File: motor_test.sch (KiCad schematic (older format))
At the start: 41 parts, among them J1 Conn_01x02_Male, J2 Conn_01x01_Male, J3 Conn_01x01_Male, J4 Conn_01x02_Male, Q1 BC817, Q10 FR024N, Q11 BC807, Q12 BC817, Q13 BC817, Q14 BC817, Q15 BC807, Q16 BC817, Q2 BC817, Q3 BC807, Q4 BC817, Q5 BC807, Q6 BC817, Q7 FR9024N, Q8 FR024N, Q9 FR9024N

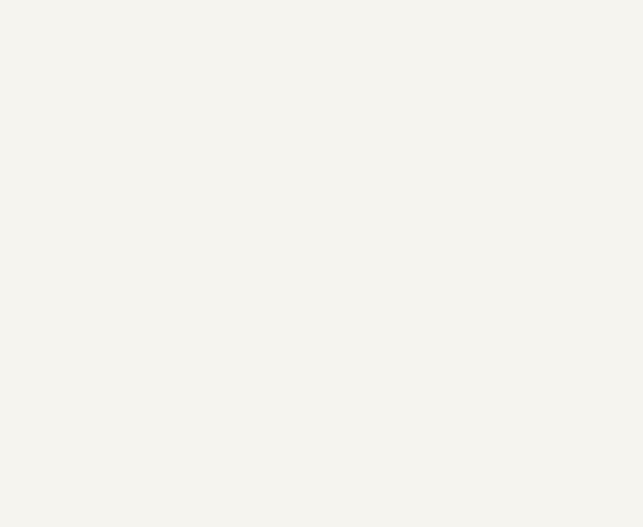
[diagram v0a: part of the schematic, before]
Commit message: bistable
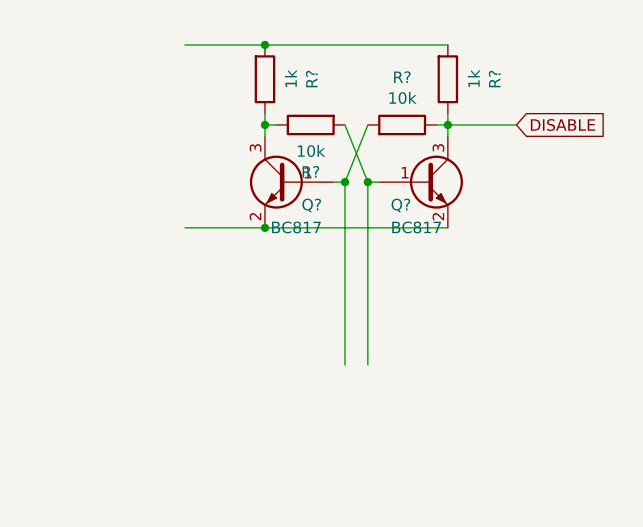
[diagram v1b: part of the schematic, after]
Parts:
- added Q? (x2): BC817, Package_TO_SOT_SMD:SOT-23, symbol Transistor_BJT:BC817
- added R? (x2): 1k, Resistor_SMD:R_1206_3216Metric, symbol Device:R
- added R? (x2): 10k, Resistor_SMD:R_1206_3216Metric, symbol Device:R
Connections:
- wire segments 119 -> 136
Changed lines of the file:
@@
 Wire Wire Line
 	1500 2550 1500 2650
+$Comp
+L Transistor_BJT:BC817 Q?
+U 1 1 5E4C4BC3
+P 8450 2450
+F 0 "Q?" H 8300 2350 50  0000 L CNN
+F 1 "BC817" H 8300 2250 50  0000 L CNN
+F 2 "Package_TO_SOT_SMD:SOT-23" H 8650 2375 50  0001 L CIN
+F 3 "http://www.fairchildsemi.com/ds/BC/BC817.pdf" H 8450 2450 50  0001 L CNN
+	1    8450 2450
+	-1   0    0    -1
+$EndComp
+$Comp
+L Transistor_BJT:BC817 Q?
+U 1 1 5E4C4F85
+P 9050 2450
+F 0 "Q?" H 8900 2350 50  0000 L CNN
+F 1 "BC817" H 8900 2250 50  0000 L CNN
+F 2 "Package_TO_SOT_SMD:SOT-23" H 9250 2375 50  0001 L CIN
+F 3 "http://www.fairchildsemi.com/ds/BC/BC817.pdf" H 9050 2450 50  0001 L CNN
+	1    9050 2450
+	1    0    0    -1
+$EndComp
+$Comp
+L Device:R R?
+U 1 1 5E4C96B6
+P 8550 2200
+F 0 "R?" V 8757 2200 50  0000 C CNN
+F 1 "10k" V 8666 2200 50  0000 C CNN
+F 2 "Resistor_SMD:R_1206_3216Metric" V 8480 2200 50  0001 C CNN
+F 3 "~" H 8550 2200 50  0001 C CNN
+	1    8550 2200
+	0    -1   1    0
+$EndComp
+$Comp
+L Device:R R?
+U 1 1 5E4C9969
+P 8950 2200
+F 0 "R?" V 9157 2200 50  0000 C CNN
+F 1 "10k" V 9066 2200 50  0000 C CNN
+F 2 "Resistor_SMD:R_1206_3216Metric" V 8880 2200 50  0001 C CNN
+F 3 "~" H 8950 2200 50  0001 C CNN
+	1    8950 2200
+	0    1    -1   0
+$EndComp
+Connection ~ 9150 2200
+Wire Wire Line
+	8700 2200 8800 2450
+Wire Wire Line
+	8800 2200 8700 2450
+Wire Wire Line
+	8700 2450 8700 3250
+Wire Wire Line
+	8800 2450 8800 3250
+Wire Wire Line
+	9150 2200 9450 2200
+Wire Wire Line
+	8350 2650 9150 2650
+Wire Wire Line
+	9150 2250 9150 2200
+Wire Wire Line
+	8350 1850 9150 1850
+$Comp
+L Device:R R?
+U 1 1 5E4C9332
+P 9150 2000
+F 0 "R?" V 9357 2000 50  0000 C CNN
+F 1 "1k" V 9266 2000 50  0000 C CNN
+F 2 "Resistor_SMD:R_1206_3216Metric" V 9080 2000 50  0001 C CNN
+F 3 "~" H 9150 2000 50  0001 C CNN
+	1    9150 2000
+	1    0    0    1
+$EndComp
+$Comp
+L Device:R R?
+U 1 1 5E4C8F84
+P 8350 2000
+F 0 "R?" V 8557 2000 50  0000 C CNN
+F 1 "1k" V 8466 2000 50  0000 C CNN
+F 2 "Resistor_SMD:R_1206_3216Metric" V 8280 2000 50  0001 C CNN
+F 3 "~" H 8350 2000 50  0001 C CNN
+	1    8350 2000
+	1    0    0    1
+$EndComp
+Wire Wire Line
+	9150 2200 9150 2150
+Wire Wire Line
+	8350 2150 8350 2200
+Wire Wire Line
+	8650 2450 8700 2450
+Connection ~ 8700 2450
+Wire Wire Line
+	8400 2200 8350 2200
+Connection ~ 8350 2200
+Wire Wire Line
+	8350 2200 8350 2250
+Wire Wire Line
+	9100 2200 9150 2200
+Wire Wire Line
+	8800 2450 8850 2450
+Connection ~ 8800 2450
+Text GLabel 9450 2200 2    50   Input ~ 0
+DISABLE
+Wire Wire Line
+	8000 1850 8350 1850
+Connection ~ 8350 1850
+Wire Wire Line
+	8350 2650 8000 2650
+Connection ~ 8350 2650
 $EndSCHEMATC

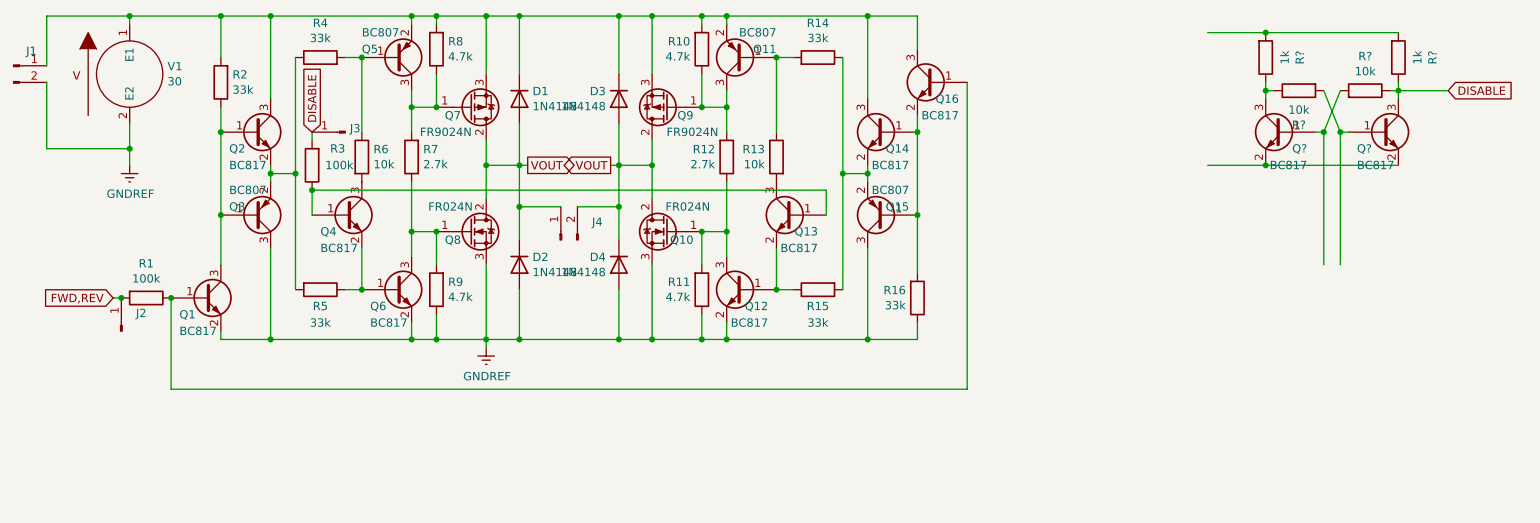
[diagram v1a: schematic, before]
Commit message: bistable
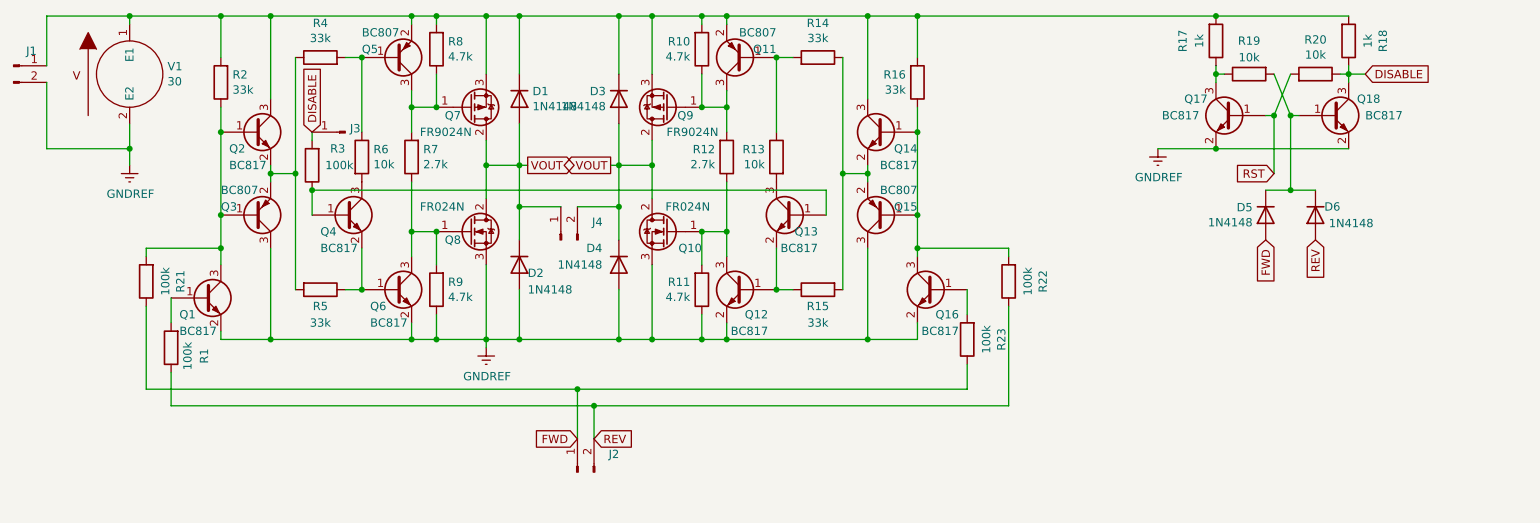
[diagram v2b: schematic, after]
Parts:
- removed J2: Conn_01x01_Male, Connector_PinHeader_2.54mm:PinHeader_1x01_P2.54mm_Vertical, symbol Connector:Conn_01x01_Male
- added D5, D6: 1N4148, Diode_THT:D_DO-35_SOD27_P7.62mm_Horizontal, symbol Diode:1N4148
- added J2: Conn_01x02_Male, Connector_PinHeader_2.54mm:PinHeader_1x02_P2.54mm_Vertical, symbol Connector:Conn_01x02_Male
- added R21, R22, R23: 100k, Resistor_SMD:R_1206_3216Metric, symbol Device:R
- gave numbers to parts that had none: 6
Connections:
- net labels added: FWD, REV, RST
- net labels removed: FWD,REV
- wire segments 136 -> 152
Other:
- moved on the sheet: Q16, Q17, Q18, R1, R16, R17, R18, R19, R20

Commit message: nightly
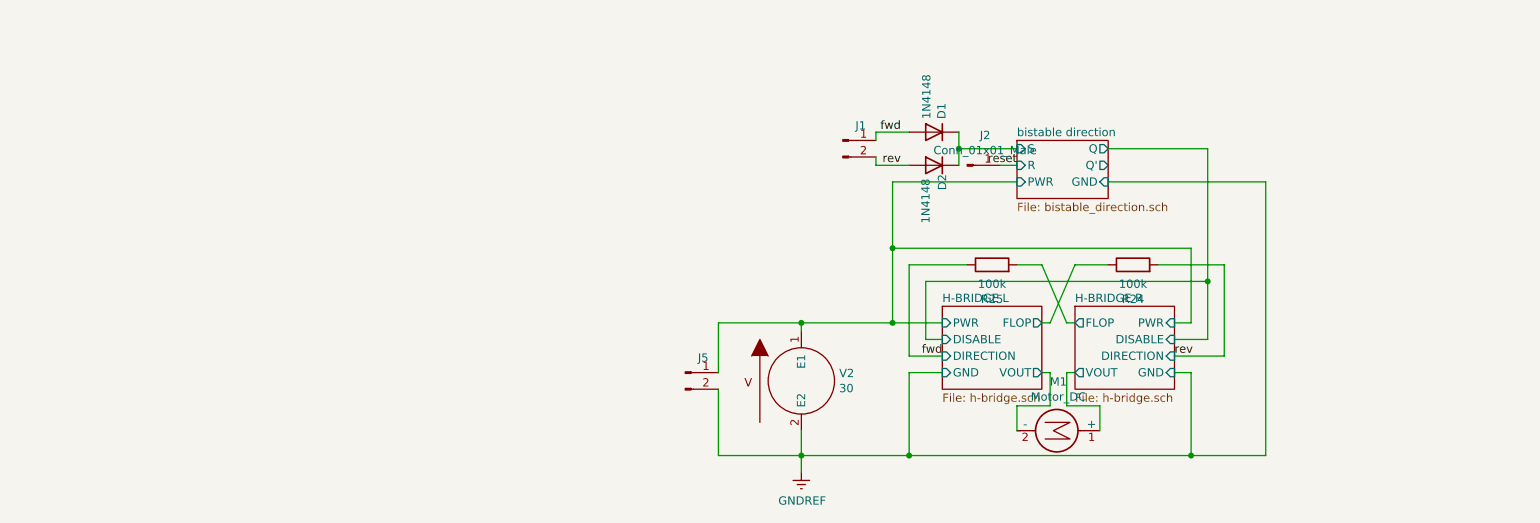
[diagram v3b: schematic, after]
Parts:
- removed D3, D4, D5, D6: 1N4148, Diode_THT:D_DO-35_SOD27_P7.62mm_Horizontal, symbol Diode:1N4148
- removed J2, J4: Conn_01x02_Male, Connector_PinHeader_2.54mm:PinHeader_1x02_P2.54mm_Vertical, symbol Connector:Conn_01x02_Male
- removed J3: Conn_01x01_Male, Connector_PinHeader_2.54mm:PinHeader_1x01_P2.54mm_Vertical, symbol Connector:Conn_01x01_Male
- removed Q1, Q12, Q13, Q14, Q16, Q17, Q18, Q2, Q4, Q6: BC817, Package_TO_SOT_SMD:SOT-23, symbol Transistor_BJT:BC817
- removed Q10, Q8: FR024N, Package_TO_SOT_SMD:TO-252-3_TabPin2, symbol Transistor_FET:FR024N
- removed Q11, Q15, Q3, Q5: BC807, Package_TO_SOT_SMD:SOT-23, symbol Transistor_BJT:BC807
- removed Q7, Q9: FR9024N, Package_TO_SOT_SMD:TO-252-3_TabPin2, symbol Transistor_FET:FR9024N
- removed R1, R21, R22, R23, R3: 100k, Resistor_SMD:R_1206_3216Metric, symbol Device:R
- removed R10, R11, R8, R9: 4.7k, Resistor_SMD:R_1206_3216Metric, symbol Device:R
- removed R12, R7: 2.7k, Resistor_SMD:R_1206_3216Metric, symbol Device:R
- removed R13, R19, R20, R6: 10k, Resistor_SMD:R_1206_3216Metric, symbol Device:R
- removed R14, R15, R16, R2, R4, R5: 33k, Resistor_SMD:R_1206_3216Metric, symbol Device:R
- removed R17, R18: 1k, Resistor_SMD:R_1206_3216Metric, symbol Device:R
- removed V1: 30, symbol pspice:VSOURCE
- added J2: Conn_01x01_Male, symbol Connector:Conn_01x01_Male
- added J5: Conn_01x02_Male, Connector_PinHeader_2.54mm:PinHeader_1x02_P2.54mm_Vertical, symbol Connector:Conn_01x02_Male
- added M1: Motor_DC, symbol Motor:Motor_DC
- added R24, R25: 100k, Resistor_SMD:R_1206_3216Metric, symbol Device:R
- added V2: 30, symbol pspice:VSOURCE
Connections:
- net GNDREF: now also J5.2 (Pin_2), V2.2 (E2); no longer D2.2 (A), J1.2 (Pin_2)
- net bistable direction/S: now reaches D1.1 (K)
- net bistable direction/S: now also D2.1 (K); no longer J1.1 (Pin_1)
- net VOUT renamed fwd
- net fwd: now also J1.1 (Pin_1), R25.1; no longer D2.1 (K)
- new net H-BRIDGE L/FLOP: R24.1
- new net H-BRIDGE L/PWR: J5.1 (Pin_1), V2.1 (E1)
- new net H-BRIDGE L/VOUT: M1.2 (-)
- new net H-BRIDGE R/FLOP: R25.2
- new net H-BRIDGE R/VOUT: M1.1 (+)
- new net reset: J2.1 (Pin_1)
- new net rev: D2.2 (A), J1.2 (Pin_2), R24.2
